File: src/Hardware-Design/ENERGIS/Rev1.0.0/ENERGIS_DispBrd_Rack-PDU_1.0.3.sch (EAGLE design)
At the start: 75 parts, among them CON1 DNI, CON2 AFC11-S20ICC-00, IC1 MCP23017T-E/ML, IC2 MCP23017T-E/ML, T1 BSS138

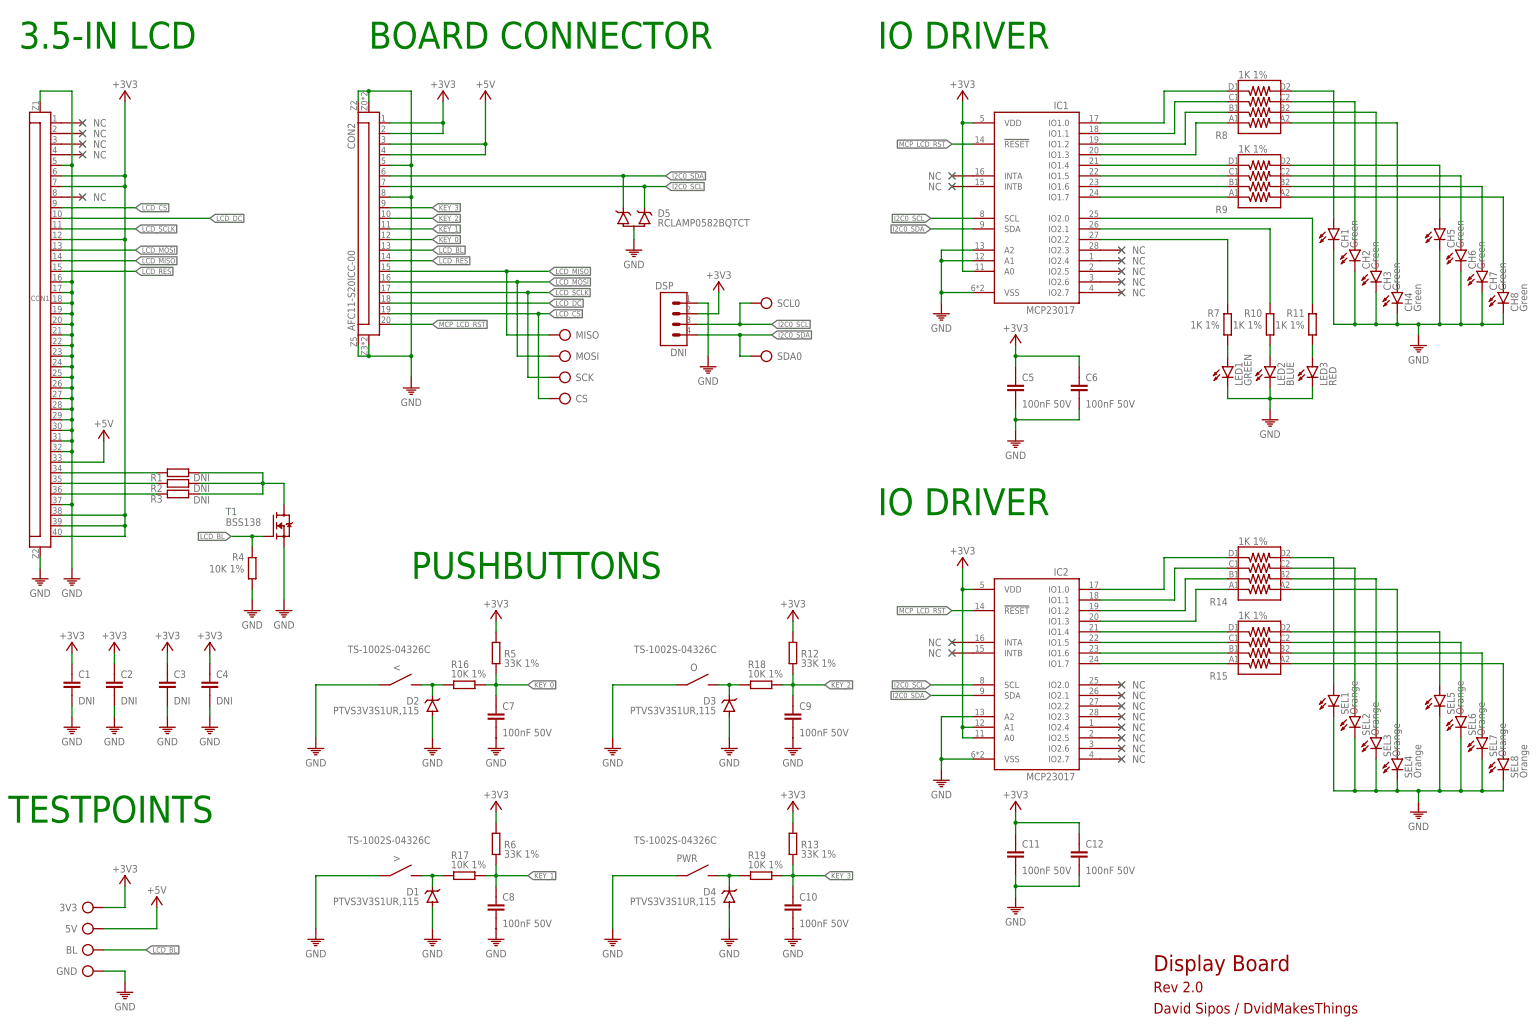
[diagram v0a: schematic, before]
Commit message: update documentation
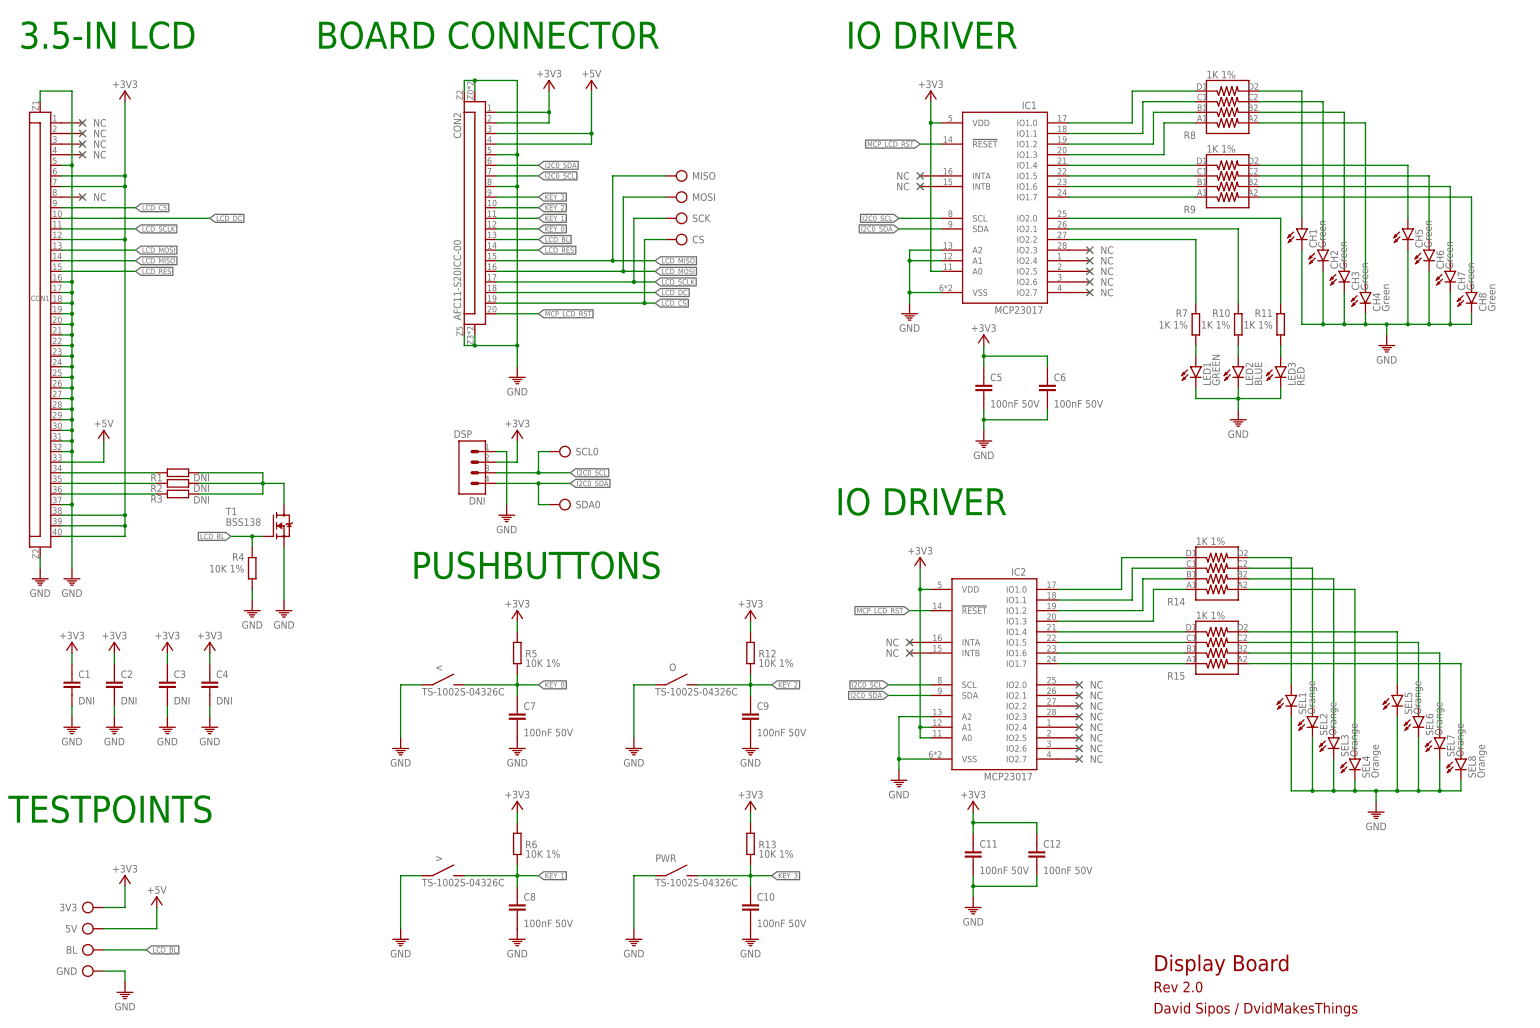
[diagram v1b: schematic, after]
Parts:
- removed D1, D2, D3, D4: PTVS3V3S1UR,115, ds_diode:PTVS3V3S1UR,115
- removed D5: RCLAMP0582BQTCT, ds_diode:RCLAMP0582BQTCT
- removed R16, R17, R18, R19: 10K 1%, ds_resistor:10K-1%0402
- R12, R13, R5, R6: value 33K 1% -> 10K 1%; device ds_resistor:33K-1%0402 -> ds_resistor:10K-1%0402
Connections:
- removed net N$24: D3.C, O.P$2, R18.1
- removed net N$25: D4.C, PWR.P$2, R19.1
- removed net N$26: >.P$2, D1.C, R17.1
- removed net N$7: <.P$2, D2.C, R16.1
- net GND: no longer D1.A, D2.A, D3.A, D4.A, D5.3
- net I2C0_SCL: no longer D5.1
- net I2C0_SDA: no longer D5.2
- net KEY_0: now also <.P$2; no longer R16.2
- net KEY_1: now also >.P$2; no longer R17.2
- net KEY_2: now also O.P$2; no longer R18.2
- net KEY_3: now also PWR.P$2; no longer R19.2
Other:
- moved on the sheet: <, >, C10, C11, C12, C5, C6, C7, C8, C9, CH1, CH2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
